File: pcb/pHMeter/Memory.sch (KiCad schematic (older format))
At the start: 5 parts, among them U7 SST25VF064C

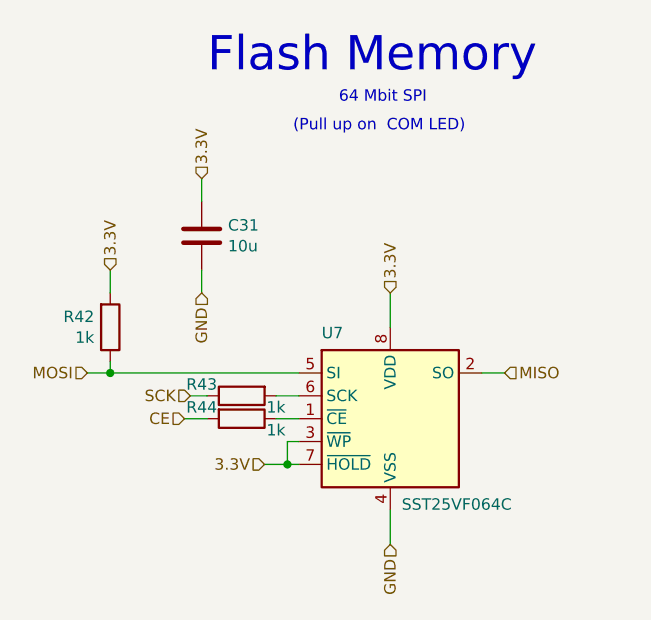
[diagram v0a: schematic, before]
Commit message: update pcb
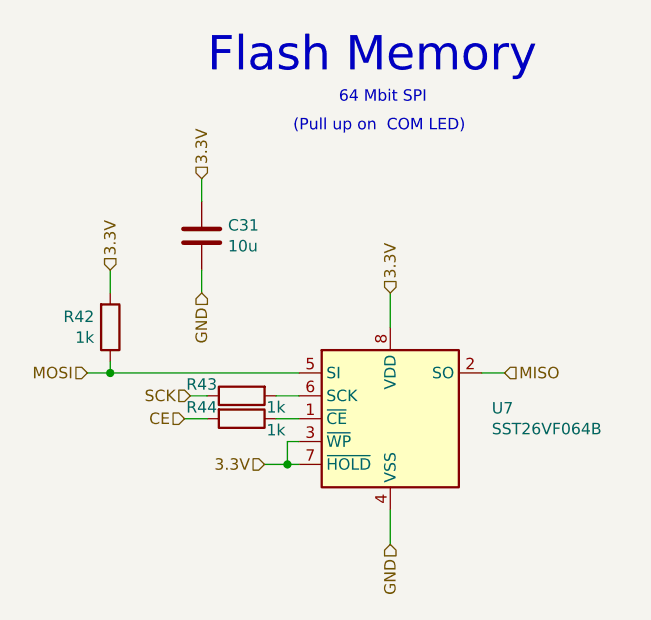
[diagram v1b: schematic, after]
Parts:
- removed U7: SST25VF064C, Package_SO:SOIC-16W_7.5x10.3mm_P1.27mm, symbol bioreactor:SST25VF064C
- added U7: SST26VF064B, Package_SO:SOIJ-8_5.3x5.3mm_P1.27mm, symbol bioreactor:SST26VF064B
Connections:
- net 3.3V: now also U7.3 (~WP~), U7.7 (~HOLD~), U7.8 (VDD)
- net GND: now also U7.4 (VSS)
- net MISO: now also U7.2 (SO)
- net MOSI: now also U7.5 (SI)
- net at R44.1: now also U7.1 (~CE)
- net at R43.2: now also U7.6 (SCK)
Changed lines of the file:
@@
 Text Notes 5025 950  0    50   ~ 0
 64 Mbit SPI
-$Comp
-L bioreactor:SST25VF064C U7
-U 1 1 5EDC79A8
-P 5250 2325
-F 0 "U7" H 4950 2700 50  0000 L CNN
-F 1 "SST25VF064C" H 5300 1950 50  0000 L CNN
-F 2 "Package_SO:SOIC-16W_7.5x10.3mm_P1.27mm" H 5250 1625 50  0001 C CNN
-F 3 "http://ww1.microchip.com/downloads/en/DeviceDoc/20005045C.pdf" H 5200 2875 50  0001 C CNN
-	1    5250 2325
-	1    0    0    -1
-$EndComp
 Text HLabel 4700 2525 0    50   Input ~ 0
 3.3V
@@
 Wire Wire Line
 	4800 2525 4700 2525
+$Comp
+L bioreactor:SST26VF064B U7
+U 1 1 5EE1E2FB
+P 5250 2325
+F 0 "U7" H 5694 2371 50  0000 L CNN
+F 1 "SST26VF064B" H 5694 2280 50  0000 L CNN
+F 2 "Package_SO:SOIJ-8_5.3x5.3mm_P1.27mm" H 5250 1625 50  0001 C CNN
+F 3 "http://ww1.microchip.com/downloads/en/DeviceDoc/SST26VF064B-SST26VF064BA-2.5V-3.0V-64-Mbit-Serial-Quad-IO-Flash-Memory-Data-Sheet-DS20005119J.pdf" H 5200 2875 50  0001 C CNN
+	1    5250 2325
+	1    0    0    -1
+$EndComp
 $EndSCHEMATC
